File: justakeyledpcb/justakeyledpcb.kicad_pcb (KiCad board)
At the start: 2 copper layers, 84.3 x 43 mm, 16 parts, among them SW1 SW_Push, SW2 SW_Push, SW3 SW_Push, SW4 SW_Push, U1 XIAO-RP2040-DIP

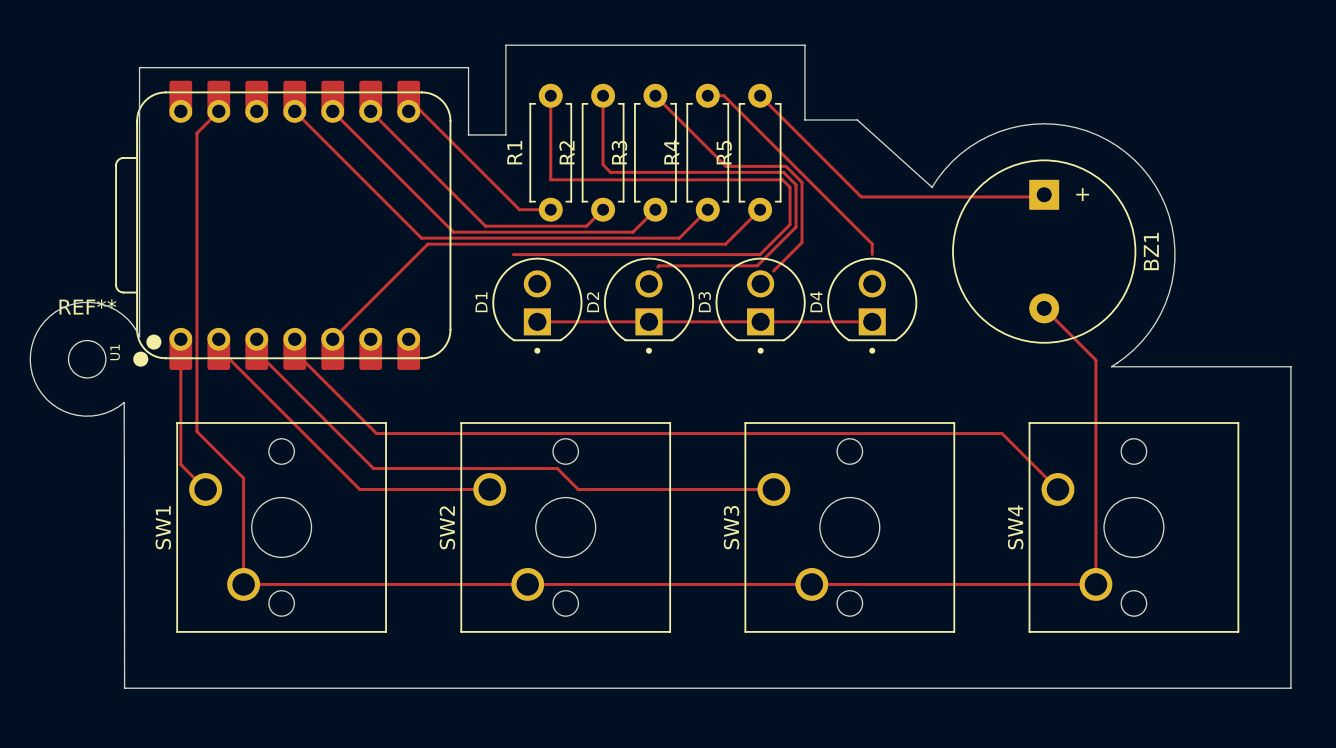
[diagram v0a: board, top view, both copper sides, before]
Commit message: FInalised the PCB Schematics and PCB Layout
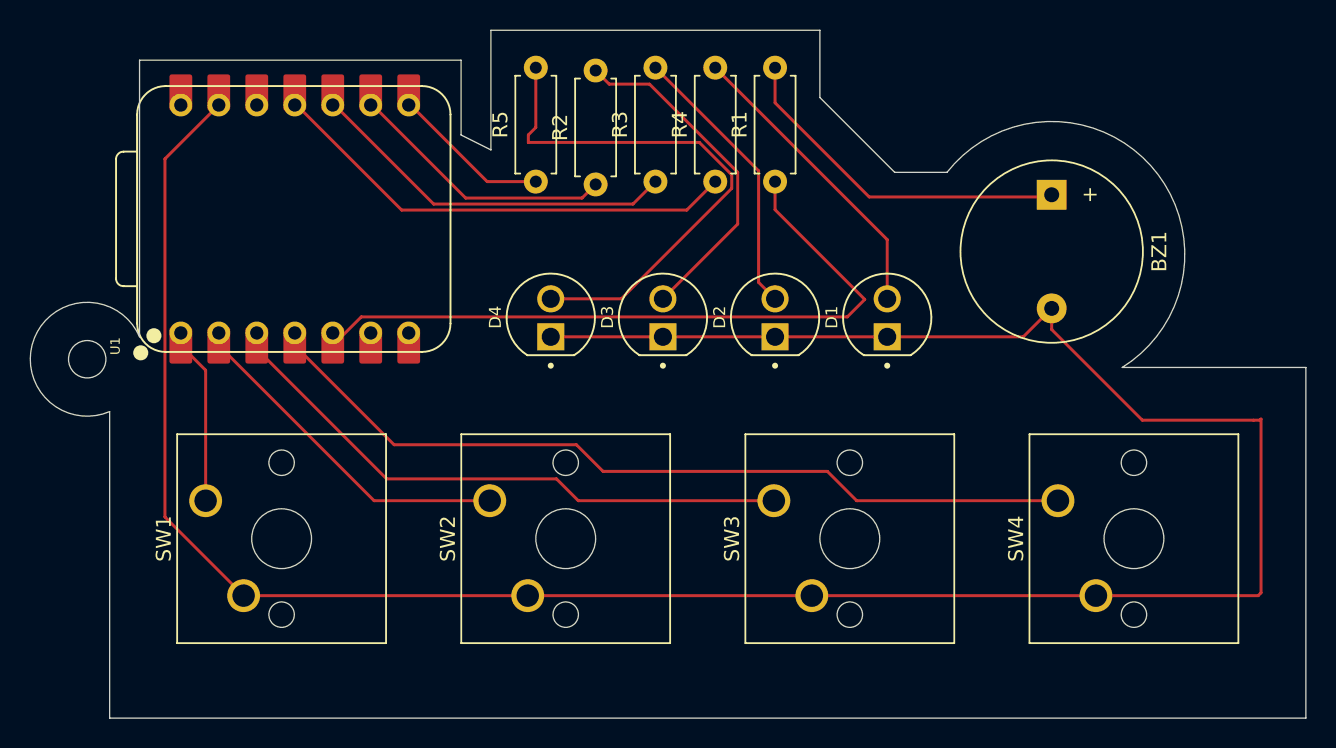
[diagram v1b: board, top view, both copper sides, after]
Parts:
- D1, D2, D3, D4: value LED -> L08R5000Q1; footprint footprints:LEDRD254W57D500H1070 -> e390cee6c564169ed6d49fe7a268946ec8897500_l08r5000q1:LEDRD254W57D500H1070
- moved D1 23.4 mm to (150.5, 58.2)
- moved D4 21.5 mm to (128.0, 58.2)
- moved R1 15.1 mm to (143.0, 49.1)
- moved R5 15.1 mm to (127.0, 49.1)
- moved D2 8.49 mm to (143.0, 58.2)
- moved D3 6.61 mm to (135.5, 58.2)
- moved R4 1.95 mm to (139.0, 49.1)
- moved R3 1.88 mm to (135.0, 49.1)
- moved R2 1.76 mm to (131.0, 49.3)
- moved SW1 0.75 mm to (104.9, 70.5)
- moved SW2 0.75 mm to (123.9, 70.5)
- moved SW3 0.75 mm to (142.9, 70.5)
- moved SW4 0.75 mm to (161.9, 70.5)
- moved BZ1 0.50 mm to (161.5, 50.0)
- moved U1 0.43 mm to (110.9, 51.6)
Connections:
- D1 pad A: (no net) -> Net-(D1-PadA)
- D1 pad C: (no net) -> GND
- D2 pad A: (no net) -> Net-(D2-PadA)
- D2 pad C: (no net) -> GND
- D3 pad A: (no net) -> Net-(D3-PadA)
- D3 pad C: (no net) -> GND
- D4 pad A: (no net) -> Net-(D4-PadA)
- D4 pad C: (no net) -> GND
- R1 pad 1: LED 1 -> Buzzer
- R1 pad 2: Net-(D1-A) -> Net-(BZ1-+)
- R2 pad 2: Net-(D2-A) -> Net-(D3-PadA)
- R3 pad 2: Net-(D3-A) -> Net-(D2-PadA)
- R4 pad 2: Net-(D4-A) -> Net-(D1-PadA)
- R5 pad 1: Buzzer -> LED 1
- R5 pad 2: Net-(BZ1-+) -> Net-(D4-PadA)
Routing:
- net GND: track 110.4 -> 168.5 mm
- net Net-(D1-A): track 43.7 -> 0.00 mm
- net Net-(D4-PadA): track 0.00 -> 35.8 mm
- net Net-(D2-A): track 31.3 -> 0.00 mm
- net Net-(D3-PadA): track 0.00 -> 22.9 mm
- net (no net): track 22.4 -> 0.00 mm
- net Net-(D1-PadA): track 0.00 -> 20.2 mm
- net Net-(D3-A): track 18.9 -> 0.00 mm
- net Net-(D2-PadA): track 0.00 -> 18.8 mm
- net Net-(D4-A): track 15.8 -> 0.00 mm
- net Buzzer: track 33.2 -> 47.2 mm
- net LED 1: track 12.6 -> 10.8 mm
- net Net-(BZ1-+): track 21.9 -> 23.5 mm
- net Button 3: track 38.4 -> 39.9 mm
- net LED 2: track 19.2 -> 18.2 mm
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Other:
- board size 84.3 x 43 mm -> 85.3 x 46 mm
